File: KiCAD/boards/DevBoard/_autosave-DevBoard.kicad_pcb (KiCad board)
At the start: 2 copper layers, 4 parts, among them J1 Conn_ARM_SWD_TagConnect_TC203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, U1 STM32C092FCP6, U2 SN65HVD232QDRG4Q1, U3 STM32C092KBT6

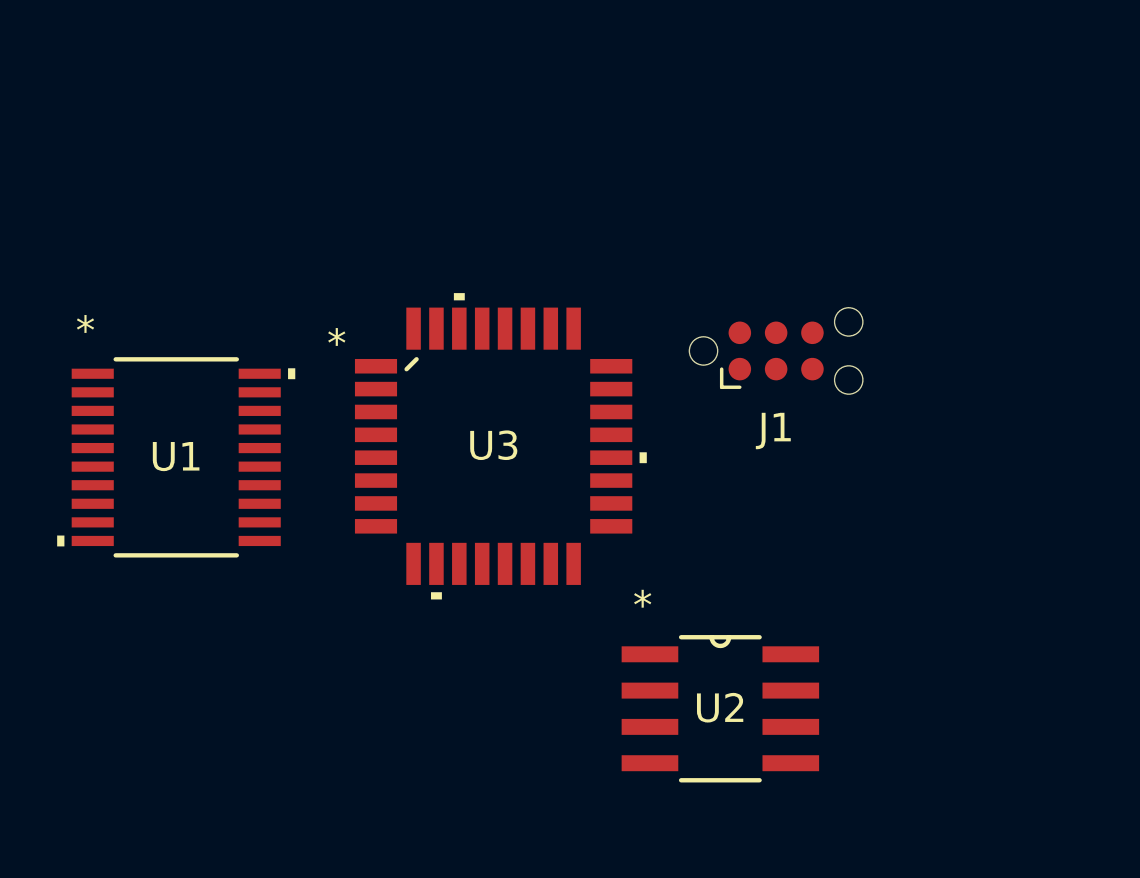
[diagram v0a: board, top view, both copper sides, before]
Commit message: DevBoard first revision
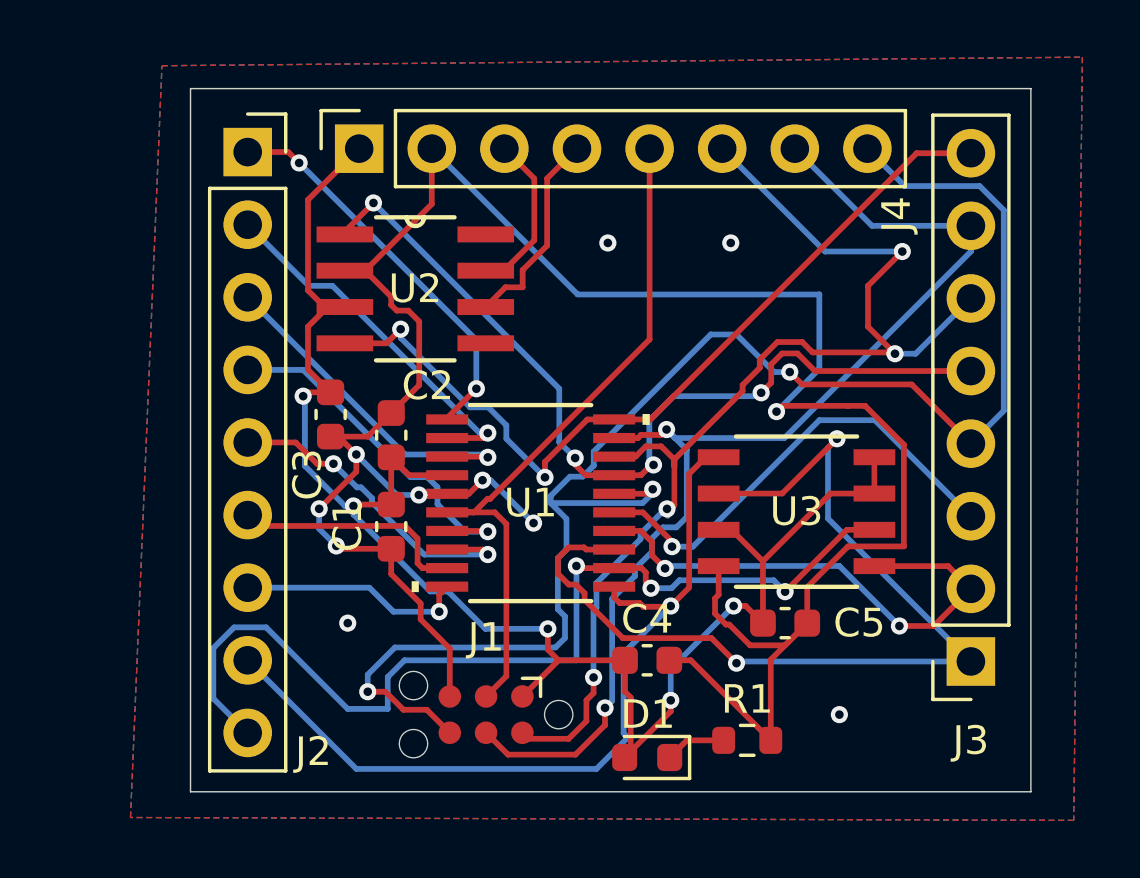
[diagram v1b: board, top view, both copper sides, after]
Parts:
- added C1: 100n, Capacitor_SMD:C_0603_1608Metric, F.Cu at (151.9, 101.9)
- added C2: 10u, Capacitor_SMD:C_0603_1608Metric, F.Cu at (151.9, 98.7)
- added C3: 100n, Capacitor_SMD:C_0603_1608Metric, F.Cu at (149.8, 98.0)
- added C4: 100n, Capacitor_SMD:C_0603_1608Metric, F.Cu at (160.9, 106.6)
- added C5: 100n, Capacitor_SMD:C_0603_1608Metric, F.Cu at (165.7, 105.3)
- added D1: LED, LED_SMD:LED_0603_1608Metric, F.Cu at (160.9, 110.0)
- added J2: Conn_01x09, Connector_PinSocket_2.54mm:PinSocket_1x09_P2.54mm_Vertical, F.Cu at (146.9, 88.8)
- added J3: Conn_01x08, Connector_PinSocket_2.54mm:PinSocket_1x08_P2.54mm_Vertical, F.Cu at (172.2, 106.6)
- added J4: Conn_01x08, Connector_PinSocket_2.54mm:PinSocket_1x08_P2.54mm_Vertical, F.Cu at (150.8, 88.7)
- added R1: 1k, Resistor_SMD:R_0603_1608Metric, F.Cu at (164.4, 109.4)
- U3: value STM32C092KBT6 -> SST25PF020B-80-4C-SAE; footprint footprints:LQFP-32_STM -> footprints:SOIC8_SA_SST_MCH
- moved U2 18.2 mm to (152.8, 93.6)
- moved J1 16.3 mm to (155.2, 108.5), turned to 180 degrees
- moved U1 12.5 mm to (156.8, 101.1)
- moved U3 10.8 mm to (166.1, 101.4)
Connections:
- U1 pad 1: unconnected-(U1-PB7/PB8-Pad1) -> /p1
- U1 pad 10: unconnected-(U1-PA3-Pad10) -> /p10
- U1 pad 11: unconnected-(U1-PA4-Pad11) -> /FLASH_CE
- U1 pad 12: unconnected-(U1-PA5-Pad12) -> /SCK
- U1 pad 13: unconnected-(U1-PA6-Pad13) -> /MISO
- U1 pad 14: unconnected-(U1-PA7-Pad14) -> /MOSI
- U1 pad 15: unconnected-(U1-PB0/PB1/PB2/PA8-Pad15) -> /p15
- U1 pad 16: unconnected-(U1-PA11[PA9]-Pad16) -> /SWO
- U1 pad 2: unconnected-(U1-PC14-OSCX_IN-Pad2) -> /p2
- U1 pad 3: unconnected-(U1-PC15-OSCX_OUT-Pad3) -> /p3
- U1 pad 6: unconnected-(U1-PF2-NRST-Pad6) -> /RESETB
- U1 pad 7: unconnected-(U1-PA0-Pad7) -> /p7
- U1 pad 8: unconnected-(U1-PA1-Pad8) -> /p8
- U1 pad 9: unconnected-(U1-PA2-Pad9) -> /p9
- U3 pad 1: unconnected-(U3-PB9-Pad1) -> /FLASH_CE
- U3 pad 2: unconnected-(U3-PC14-OSCX_IN-Pad2) -> /MISO
- U3 pad 3: unconnected-(U3-PC15-OSCX_OUT-Pad3) -> +3V3
- U3 pad 4: unconnected-(U3-VDD/VDDA-Pad4) -> GND
- U3 pad 5: unconnected-(U3-VSS/VSSA-Pad5) -> /MOSI
- U3 pad 6: unconnected-(U3-PF2-NRST-Pad6) -> /SCK
- U3 pad 7: unconnected-(U3-PA0-Pad7) -> +3V3
- U3 pad 8: unconnected-(U3-PA1-Pad8) -> +3V3
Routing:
- net GND: track 0.00 -> 84.9 mm, vias 0 -> 11
- net +3V3: track 0.00 -> 58.6 mm, vias 0 -> 5
- net /SWO: track 0.00 -> 55.4 mm, vias 0 -> 3
- net /SWDIO: track 0.00 -> 41.7 mm, vias 0 -> 4
- net /SWCLK: track 0.00 -> 40.6 mm, vias 0 -> 2
- net /SCK: track 0.00 -> 34.4 mm, vias 0 -> 3
- net /MISO: track 0.00 -> 33.5 mm, vias 0 -> 2
- net /CANTX: track 0.00 -> 31.1 mm, vias 0 -> 4
- net /CANRX: track 0.00 -> 29.7 mm, vias 0 -> 2
- net /FLASH_CE: track 0.00 -> 29.3 mm, vias 0 -> 1
- net /RESETB: track 0.00 -> 24.8 mm
- net /MOSI: track 0.00 -> 18.4 mm, vias 0 -> 2
- net /p15: track 0.00 -> 16.3 mm, vias 0 -> 1
- net /p1: track 0.00 -> 13.9 mm, vias 0 -> 2
- net /p2: track 0.00 -> 12.9 mm, vias 0 -> 1
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- added copper zone on B.Cu, net GND
- added copper zone on F.Cu, net GND
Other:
- board outline added: 29.4 x 24.6 mm
